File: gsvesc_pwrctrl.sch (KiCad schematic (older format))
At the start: 13 parts, among them Q7 NVMFS5C604, U7 LM2594HVM-5.0, U8 LT1910

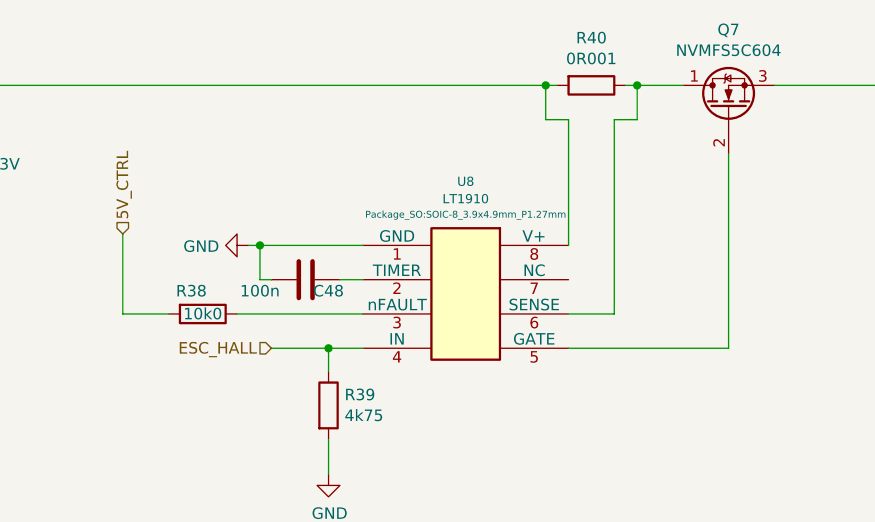
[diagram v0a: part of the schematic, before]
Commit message: design finished gerber created
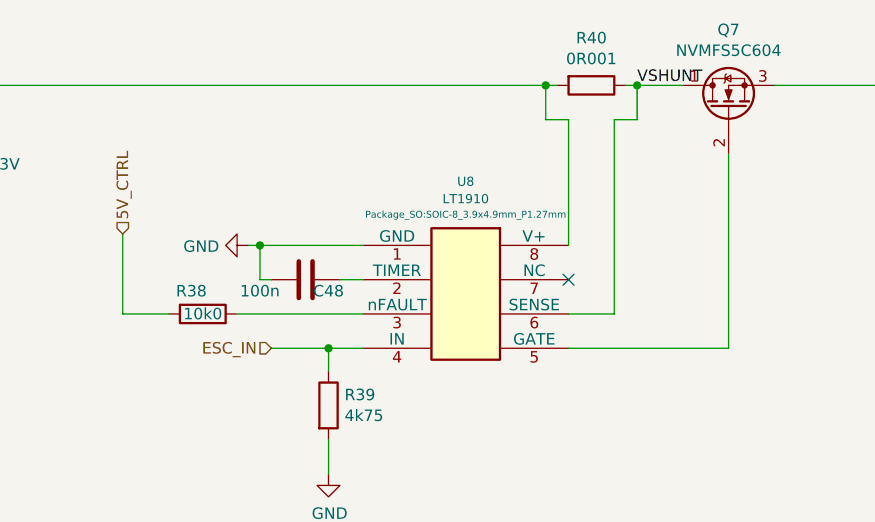
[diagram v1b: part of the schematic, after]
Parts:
- C47: footprint Capacitor_SMD:CP_Elec_16x17.5 -> Capacitor_Tantalum_SMD:CP_EIA-3216-18_Kemet-A
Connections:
- net VSHUNT: now reaches Q7.1 (D), R40.1, U8.6 (SENSE)
- net ESC_HALL renamed ESC_IN
- no-connect marks 0 -> 1
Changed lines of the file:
@@
 5V_CTRL
 Text HLabel 4300 2600 0    50   Input ~ 0
-ESC_HALL
+ESC_IN
 $Comp
 L Regulator_Switching:LM2594HVM-5.0 U7
@@
 F 0 "C47" H 4100 4550 50  0000 L CNN
 F 1 "100u/16V" H 4050 4300 50  0000 L CNN
-F 2 "Capacitor_SMD:CP_Elec_16x17.5" H 4088 4300 50  0001 C CNN
+F 2 "Capacitor_Tantalum_SMD:CP_EIA-3216-18_Kemet-A" H 4088 4300 50  0001 C CNN
 F 3 "~" H 4050 4450 50  0001 C CNN
 	1    4050 4450
@@
 	2750 4700 3250 4700
 Connection ~ 2750 4700
+Text Label 5900 1450 0    50   ~ 0
+VSHUNT
+NoConn ~ 5600 2300
 $EndSCHEMATC

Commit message: fix some bugs
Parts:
- removed R39: 4k75, Resistor_SMD:R_0805_2012Metric, symbol Device:R
- added Q?: BC856, Package_TO_SOT_SMD:SOT-23, symbol Transistor_BJT:BC856
- added R? (x2): 10k, symbol Device:R
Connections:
- wire segments 59 -> 64
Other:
- moved on the sheet: C48, Q7, R38, R40, U8
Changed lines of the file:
@@
 L gsvesc:LT1910 U8
 U 1 1 5C03A92E
-P 5150 2350
-F 0 "U8" V 4671 2350 40  0000 C CNN
-F 1 "LT1910" V 4747 2350 40  0000 C CNN
-F 2 "Package_SO:SOIC-8_3.9x4.9mm_P1.27mm" V 4815 2350 30  0000 C CNN
-F 3 "" H 5150 2350 60  0000 C CNN
-	1    5150 2350
-	0    1    1    0
-$EndComp
-Wire Wire Line
-	5900 1450 6100 1450
-Wire Wire Line
-	5600 1600 5600 2150
-Wire Wire Line
-	5600 2450 5800 2450
-Wire Wire Line
-	5800 1600 5800 2450
-Wire Wire Line
-	5600 2600 6300 2600
-Wire Wire Line
-	6300 2600 6300 1750
-Wire Wire Line
-	4700 2150 4250 2150
+P 5800 2350
+F 0 "U8" V 5321 2350 40  0000 C CNN
+F 1 "LT1910" V 5397 2350 40  0000 C CNN
+F 2 "Package_SO:SOIC-8_3.9x4.9mm_P1.27mm" V 5465 2350 30  0000 C CNN
+F 3 "" H 5800 2350 60  0000 C CNN
+	1    5800 2350
+	0    1    1    0
+$EndComp
+Wire Wire Line
+	6550 1450 6750 1450
+Wire Wire Line
+	6250 1600 6250 2150
+Wire Wire Line
+	6250 2450 6450 2450
+Wire Wire Line
+	6450 1600 6450 2450
+Wire Wire Line
+	6250 2600 6950 2600
+Wire Wire Line
+	6950 2600 6950 1750
+Wire Wire Line
+	5350 2150 4900 2150
 $Comp
 L Device:C C48
 U 1 1 5C03B687
-P 4450 2300
-F 0 "C48" V 4500 2400 50  0000 C CNN
-F 1 "100n" V 4500 2100 50  0000 C CNN
-F 2 "Capacitor_SMD:C_0805_2012Metric" H 4488 2150 50  0001 C CNN
-F 3 "~" H 4450 2300 50  0001 C CNN
-	1    4450 2300
-	0    1    1    0
-$EndComp
-Wire Wire Line
-	4700 2300 4600 2300
-Wire Wire Line
-	4300 2300 4250 2300
-Wire Wire Line
-	4250 2300 4250 2150
-Wire Wire Line
-	4250 2150 4200 2150
-Connection ~ 4250 2150
+P 5100 2300
+F 0 "C48" V 5150 2400 50  0000 C CNN
+F 1 "100n" V 5150 2100 50  0000 C CNN
+F 2 "Capacitor_SMD:C_0805_2012Metric" H 5138 2150 50  0001 C CNN
+F 3 "~" H 5100 2300 50  0001 C CNN
+	1    5100 2300
+	0    1    1    0
+$EndComp
+Wire Wire Line
+	5350 2300 5250 2300
+Wire Wire Line
+	4950 2300 4900 2300
+Wire Wire Line
+	4900 2300 4900 2150
+Wire Wire Line
+	4900 2150 4850 2150
+Connection ~ 4900 2150
 $Comp
 L power:GND #PWR061
 U 1 1 5C03BA66
-P 4200 2150
-F 0 "#PWR061" H 4200 1900 50  0001 C CNN
-F 1 "GND" V 4205 2022 50  0000 R CNN
-F 2 "" H 4200 2150 50  0001 C CNN
-F 3 "" H 4200 2150 50  0001 C CNN
-	1    4200 2150
-	0    1    1    0
-$EndComp
-Connection ~ 2750 1450
+P 4850 2150
+F 0 "#PWR061" H 4850 1900 50  0001 C CNN
+F 1 "GND" V 4855 2022 50  0000 R CNN
+F 2 "" H 4850 2150 50  0001 C CNN
+F 3 "" H 4850 2150 50  0001 C CNN
+	1    4850 2150
+	0    1    1    0
+$EndComp
 $Comp
 L Device:R R38
 U 1 1 5C03BF03
-P 4000 2450
-F 0 "R38" V 3900 2400 50  0000 C CNN
-F 1 "10k0" V 4000 2450 50  0000 C CNN
-F 2 "Resistor_SMD:R_0805_2012Metric" V 3930 2450 50  0001 C CNN
-F 3 "~" H 4000 2450 50  0001 C CNN
-	1    4000 2450
-	0    1    1    0
-$EndComp
-Wire Wire Line
-	4150 2450 4700 2450
-Wire Wire Line
-	3850 2450 3650 2450
-Wire Wire Line
-	3650 2450 3650 2100
-Wire Wire Line
-	4700 2600 4550 2600
-$Comp
-L Device:R R39
-U 1 1 5C03C608
-P 4550 2850
-F 0 "R39" H 4620 2896 50  0000 L CNN
-F 1 "4k75" H 4620 2805 50  0000 L CNN
-F 2 "Resistor_SMD:R_0805_2012Metric" V 4480 2850 50  0001 C CNN
-F 3 "~" H 4550 2850 50  0001 C CNN
-	1    4550 2850
-	1    0    0    -1
-$EndComp
-Wire Wire Line
-	4550 2700 4550 2600
-Connection ~ 4550 2600
-Wire Wire Line
-	4550 2600 4300 2600
-Wire Wire Line
-	4550 3000 4550 3150
+P 4300 2250
+F 0 "R38" H 4150 2200 50  0000 C CNN
+F 1 "10k0" H 4150 2300 50  0000 C CNN
+F 2 "Resistor_SMD:R_0805_2012Metric" V 4230 2250 50  0001 C CNN
+F 3 "~" H 4300 2250 50  0001 C CNN
+	1    4300 2250
+	-1   0    0    1
+$EndComp
 $Comp
 L power:GND #PWR062
 U 1 1 5C03CB9C
-P 4550 3150
-F 0 "#PWR062" H 4550 2900 50  0001 C CNN
-F 1 "GND" H 4555 2977 50  0000 C CNN
-F 2 "" H 4550 3150 50  0001 C CNN
-F 3 "" H 4550 3150 50  0001 C CNN
-	1    4550 3150
-	1    0    0    -1
-$EndComp
-Wire Wire Line
-	6500 1450 7150 1450
-Text HLabel 7150 1450 2    50   Input ~ 0
+P 4050 3200
+F 0 "#PWR062" H 4050 2950 50  0001 C CNN
+F 1 "GND" H 4055 3027 50  0000 C CNN
+F 2 "" H 4050 3200 50  0001 C CNN
+F 3 "" H 4050 3200 50  0001 C CNN
+	1    4050 3200
+	1    0    0    -1
+$EndComp
+Wire Wire Line
+	7150 1450 7800 1450
+Text HLabel 7800 1450 2    50   Input ~ 0
 VBAT
-Text HLabel 3650 2100 1    50   Input ~ 0
+Text HLabel 4300 1950 1    50   Input ~ 0
 5V_CTRL
-Text HLabel 4300 2600 0    50   Input ~ 0
+Text HLabel 3600 2800 0    50   Input ~ 0
 ESC_IN
 $Comp
@@
 L gsvesc:NVMFS5C604 Q7
 U 1 1 5C011119
-P 6300 1550
-F 0 "Q7" V 6643 1550 50  0000 C CNN
-F 1 "NVMFS5C604" V 6552 1550 50  0000 C CNN
-F 2 "gsvesc:DFN500X600X110-5N" H 6300 1550 50  0001 C CIN
-F 3 "" H 6300 1550 50  0001 L CNN
-	1    6300 1550
+P 6950 1550
+F 0 "Q7" V 7293 1550 50  0000 C CNN
+F 1 "NVMFS5C604" V 7202 1550 50  0000 C CNN
+F 2 "gsvesc:DFN500X600X110-5N" H 6950 1550 50  0001 C CIN
+F 3 "" H 6950 1550 50  0001 L CNN
+	1    6950 1550
 	0    -1   -1   0
 $EndComp
@@
 L Device:R R40
 U 1 1 5C118A80
-P 5700 1450
-F 0 "R40" V 5493 1450 50  0000 C CNN
-F 1 "0R001" V 5584 1450 50  0000 C CNN
-F 2 "Resistor_SMD:R_2512_6332Metric" V 5630 1450 50  0001 C CNN
-F 3 "~" H 5700 1450 50  0001 C CNN
-	1    5700 1450
-	0    1    1    0
-$EndComp
-Wire Wire Line
-	5800 1600 5900 1600
-Wire Wire Line
-	5900 1600 5900 1450
-Wire Wire Line
-	5900 1450 5850 1450
-Connection ~ 5900 1450
-Wire Wire Line
-	2750 1450 5500 1450
-Wire Wire Line
-	5500 1450 5500 1600
-Wire Wire Line
-	5500 1600 5600 1600
-Connection ~ 5500 1450
-Wire Wire Line
-	5500 1450 5550 1450
+P 6350 1450
+F 0 "R40" V 6143 1450 50  0000 C CNN
+F 1 "0R001" V 6234 1450 50  0000 C CNN
+F 2 "Resistor_SMD:R_2512_6332Metric" V 6280 1450 50  0001 C CNN
+F 3 "~" H 6350 1450 50  0001 C CNN
+	1    6350 1450
+	0    1    1    0
+$EndComp
+Wire Wire Line
+	6450 1600 6550 1600
+Wire Wire Line
+	6550 1600 6550 1450
+Wire Wire Line
+	6550 1450 6500 1450
+Connection ~ 6550 1450
+Wire Wire Line
+	2750 1450 6150 1450
+Wire Wire Line
+	6150 1450 6150 1600
+Wire Wire Line
+	6150 1600 6250 1600
+Connection ~ 6150 1450
+Wire Wire Line
+	6150 1450 6200 1450
 Wire Wire Line
 	2750 4700 3250 4700
 Connection ~ 2750 4700
-Text Label 5900 1450 0    50   ~ 0
+Text Label 6550 1450 0    50   ~ 0
 VSHUNT
-NoConn ~ 5600 2300
+NoConn ~ 6250 2300
+Wire Wire Line
+	5350 2450 4300 2450
+Wire Wire Line
+	4300 2450 4300 2400
+Wire Wire Line
+	4300 2100 4300 2000
+$Comp
+L Device:R R?
+U 1 1 5C6C221A
+P 4050 2250
+F 0 "R?" H 4120 2296 50  0000 L CNN
+F 1 "10k" H 4120 2205 50  0000 L CNN
+F 2 "" V 3980 2250 50  0001 C CNN
+F 3 "~" H 4050 2250 50  0001 C CNN
+	1    4050 2250
+	1    0    0    -1
+$EndComp
+$Comp
+L Device:R R?
+U 1 1 5C6C2297
+P 3750 2300
+F 0 "R?" H 3820 2346 50  0000 L CNN
+F 1 "10k" H 3820 2255 50  0000 L CNN
+F 2 "" V 3680 2300 50  0001 C CNN
+F 3 "~" H 3750 2300 50  0001 C CNN
+	1    3750 2300
+	1    0    0    -1
+$EndComp
+Wire Wire Line
+	3750 2150 3750 2000
+Wire Wire Line
+	3750 2000 4300 2000
+Connection ~ 4300 2000
+Wire Wire Line
+	4300 2000 4300 1950
+Wire Wire Line
+	4050 2100 4300 2100
+Connection ~ 4300 2100
+Connection ~ 2750 1450
+Wire Wire Line
+	4050 2400 4050 2600
+Wire Wire Line
+	4050 2600 5350 2600
+$Comp
+L Transistor_BJT:BC856 Q?
+U 1 1 5C6CACEB
+P 3950 2800
+F 0 "Q?" H 4141 2846 50  0000 L CNN
+F 1 "BC856" H 4141 2755 50  0000 L CNN
+F 2 "Package_TO_SOT_SMD:SOT-23" H 4150 2725 50  0001 L CIN
+F 3 "http://www.fairchildsemi.com/ds/BC/BC856.pdf" H 3950 2800 50  0001 L CNN
+	1    3950 2800
+	1    0    0    -1
+$EndComp
+Connection ~ 4050 2600
+Wire Wire Line
+	4050 3000 4050 3200
+Wire Wire Line
+	3750 2450 3750 2800
+Wire Wire Line
+	3600 2800 3750 2800
+Connection ~ 3750 2800
 $EndSCHEMATC

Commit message: change inverter to npn :)
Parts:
- removed Q?: BC856, Package_TO_SOT_SMD:SOT-23, symbol Transistor_BJT:BC856
- added Q?: BC847, Package_TO_SOT_SMD:SOT-23, symbol Transistor_BJT:BC847
- Q7: symbol gsvesc:NVMFS5C604 -> gsvesc-rescue:NVMFS5C604-gsvesc
- U8: symbol gsvesc:LT1910 -> gsvesc-rescue:LT1910-gsvesc
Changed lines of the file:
@@
 $EndComp
 $Comp
-L gsvesc:LT1910 U8
+L gsvesc-rescue:LT1910-gsvesc U8
 U 1 1 5C03A92E
 P 5800 2350
@@
 Power Control
 $Comp
-L gsvesc:NVMFS5C604 Q7
+L gsvesc-rescue:NVMFS5C604-gsvesc Q7
 U 1 1 5C011119
 P 6950 1550
@@
 Wire Wire Line
 	4050 2600 5350 2600
-$Comp
-L Transistor_BJT:BC856 Q?
-U 1 1 5C6CACEB
+Wire Wire Line
+	4050 3000 4050 3200
+Wire Wire Line
+	3750 2450 3750 2800
+Wire Wire Line
+	3600 2800 3750 2800
+$Comp
+L Transistor_BJT:BC847 Q?
+U 1 1 5C6C04CF
 P 3950 2800
 F 0 "Q?" H 4141 2846 50  0000 L CNN
-F 1 "BC856" H 4141 2755 50  0000 L CNN
+F 1 "BC847" H 4141 2755 50  0000 L CNN
 F 2 "Package_TO_SOT_SMD:SOT-23" H 4150 2725 50  0001 L CIN
-F 3 "http://www.fairchildsemi.com/ds/BC/BC856.pdf" H 3950 2800 50  0001 L CNN
+F 3 "http://www.infineon.com/dgdl/Infineon-BC847SERIES_BC848SERIES_BC849SERIES_BC850SERIES-DS-v01_01-en.pdf?fileId=db3a304314dca389011541d4630a1657" H 3950 2800 50  0001 L CNN
 	1    3950 2800
 	1    0    0    -1
 $EndComp
+Connection ~ 3750 2800
 Connection ~ 4050 2600
-Wire Wire Line
-	4050 3000 4050 3200
-Wire Wire Line
-	3750 2450 3750 2800
-Wire Wire Line
-	3600 2800 3750 2800
-Connection ~ 3750 2800
 $EndSCHEMATC
